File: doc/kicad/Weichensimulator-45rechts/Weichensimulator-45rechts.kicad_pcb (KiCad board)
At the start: 2 copper layers, 38.1 x 38.1 mm, 10 parts, among them J1 Conn_01x02_Male, J2 Power, J3 Conn_01x02_Male, K1 HFD2_005-S-L2-D

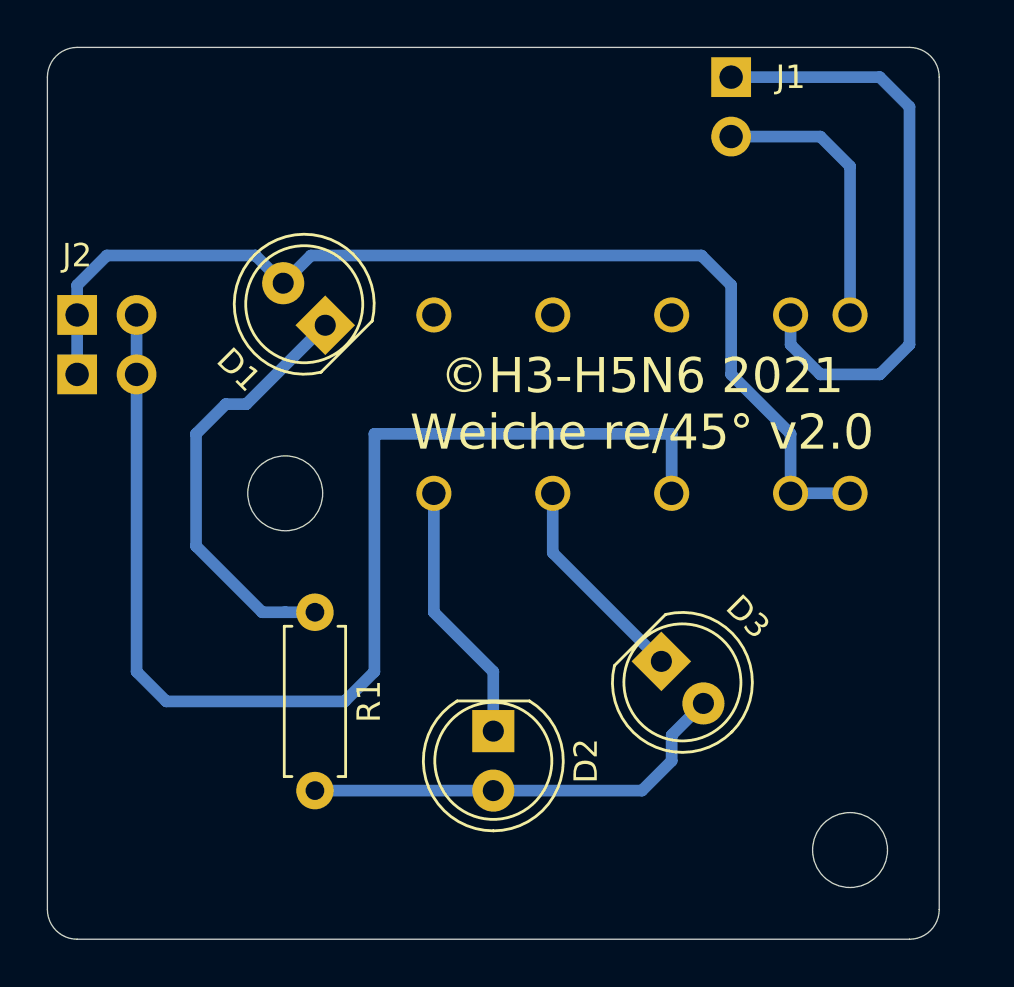
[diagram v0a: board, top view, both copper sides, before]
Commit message: Dateien aufgeräumt
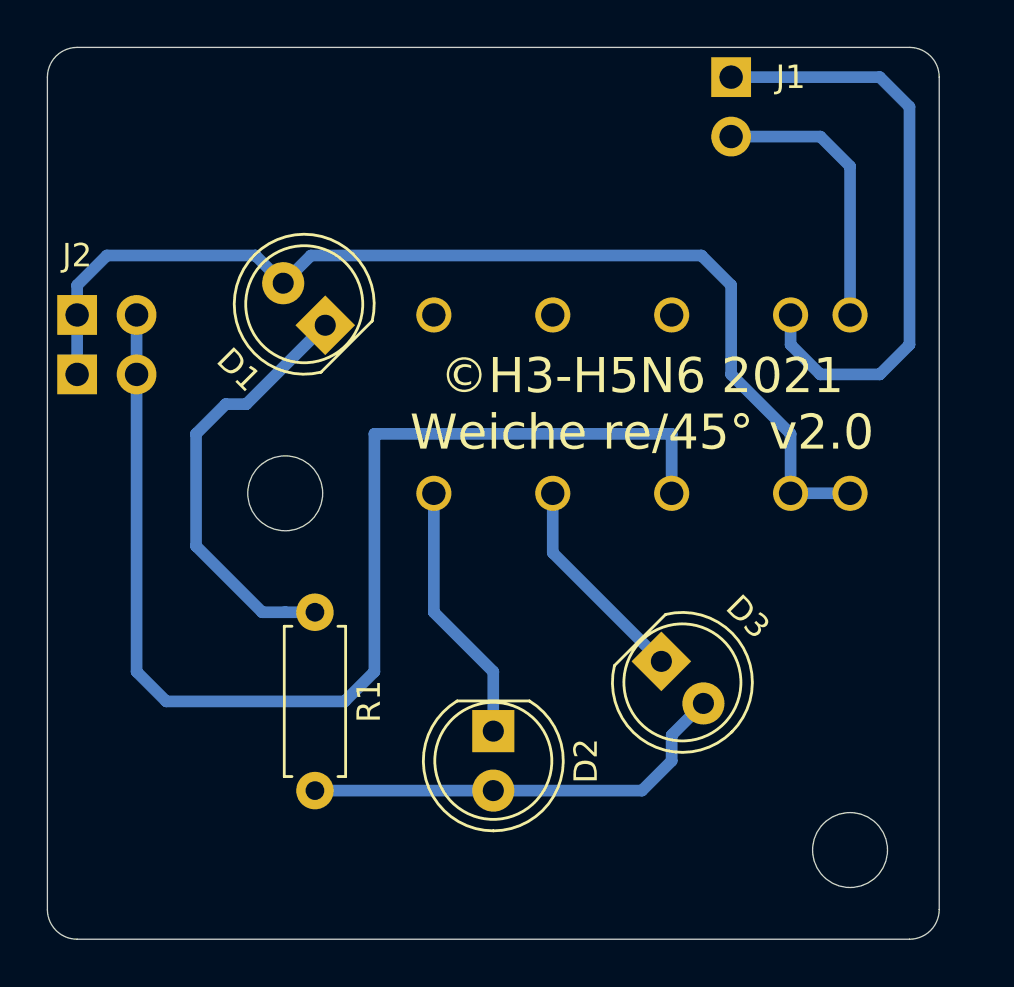
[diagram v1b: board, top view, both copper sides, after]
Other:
- net class Default removed
